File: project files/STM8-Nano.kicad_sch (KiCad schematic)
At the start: 29 parts, among them J1 RIGHT, J2 LEFT, J3 USB_C_Receptacle, J4 SWIM, SW1 RESET, SW2 VCC, U1 STM8F105K4, U2 CH340E, Y1 16MHZ

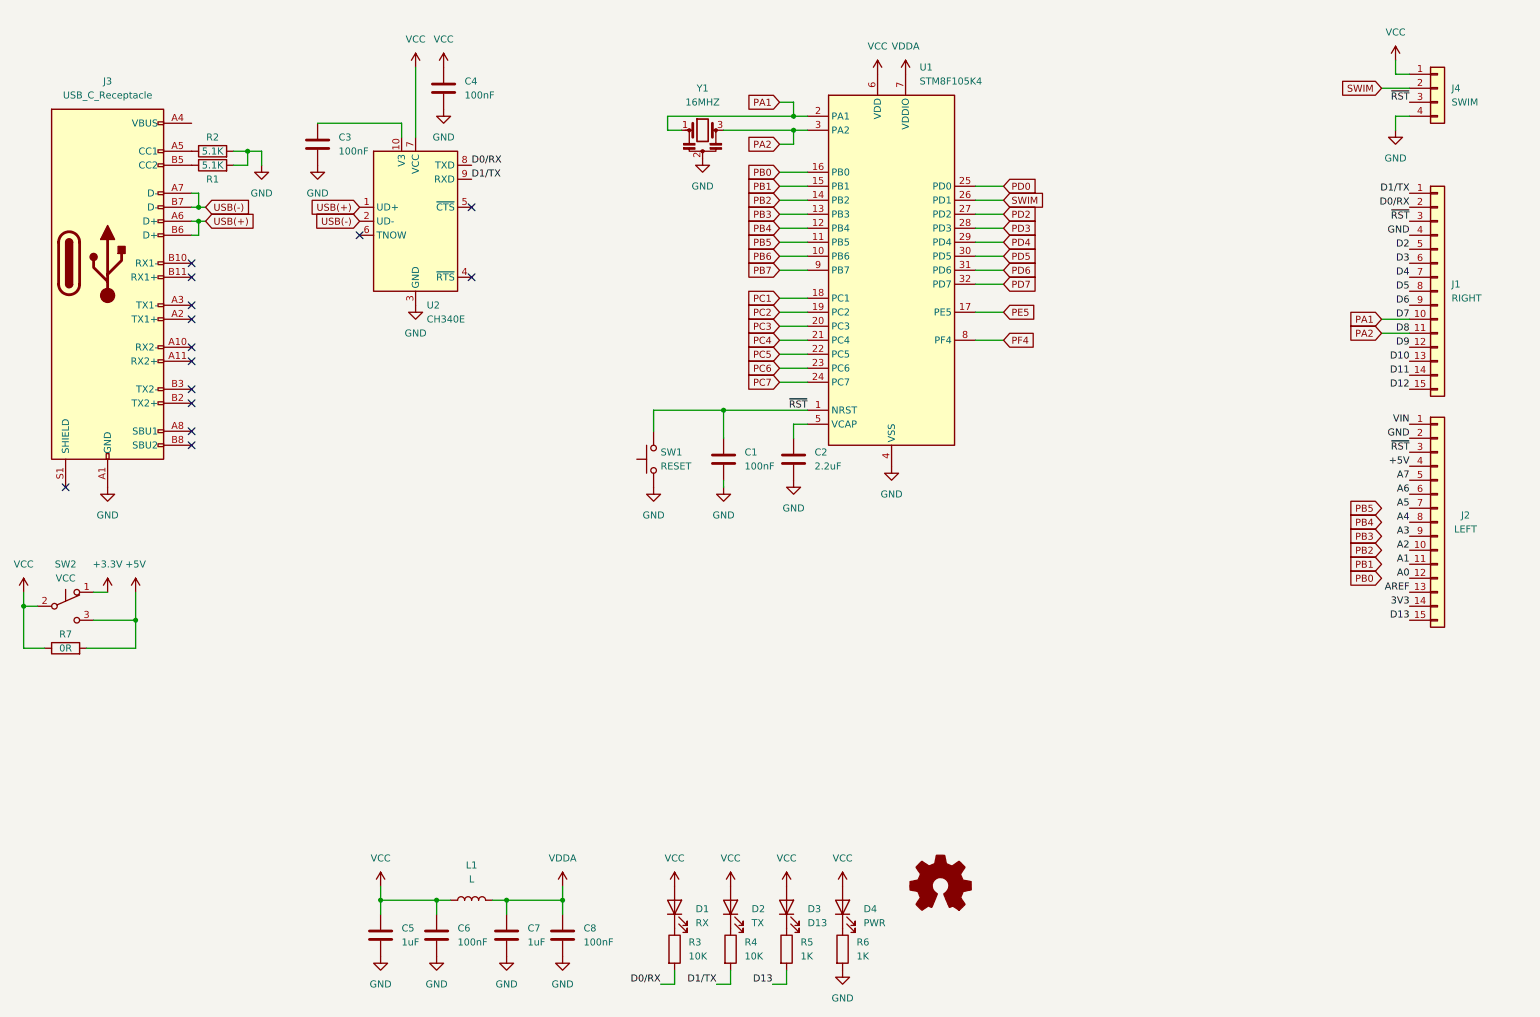
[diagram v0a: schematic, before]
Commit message: added annotation
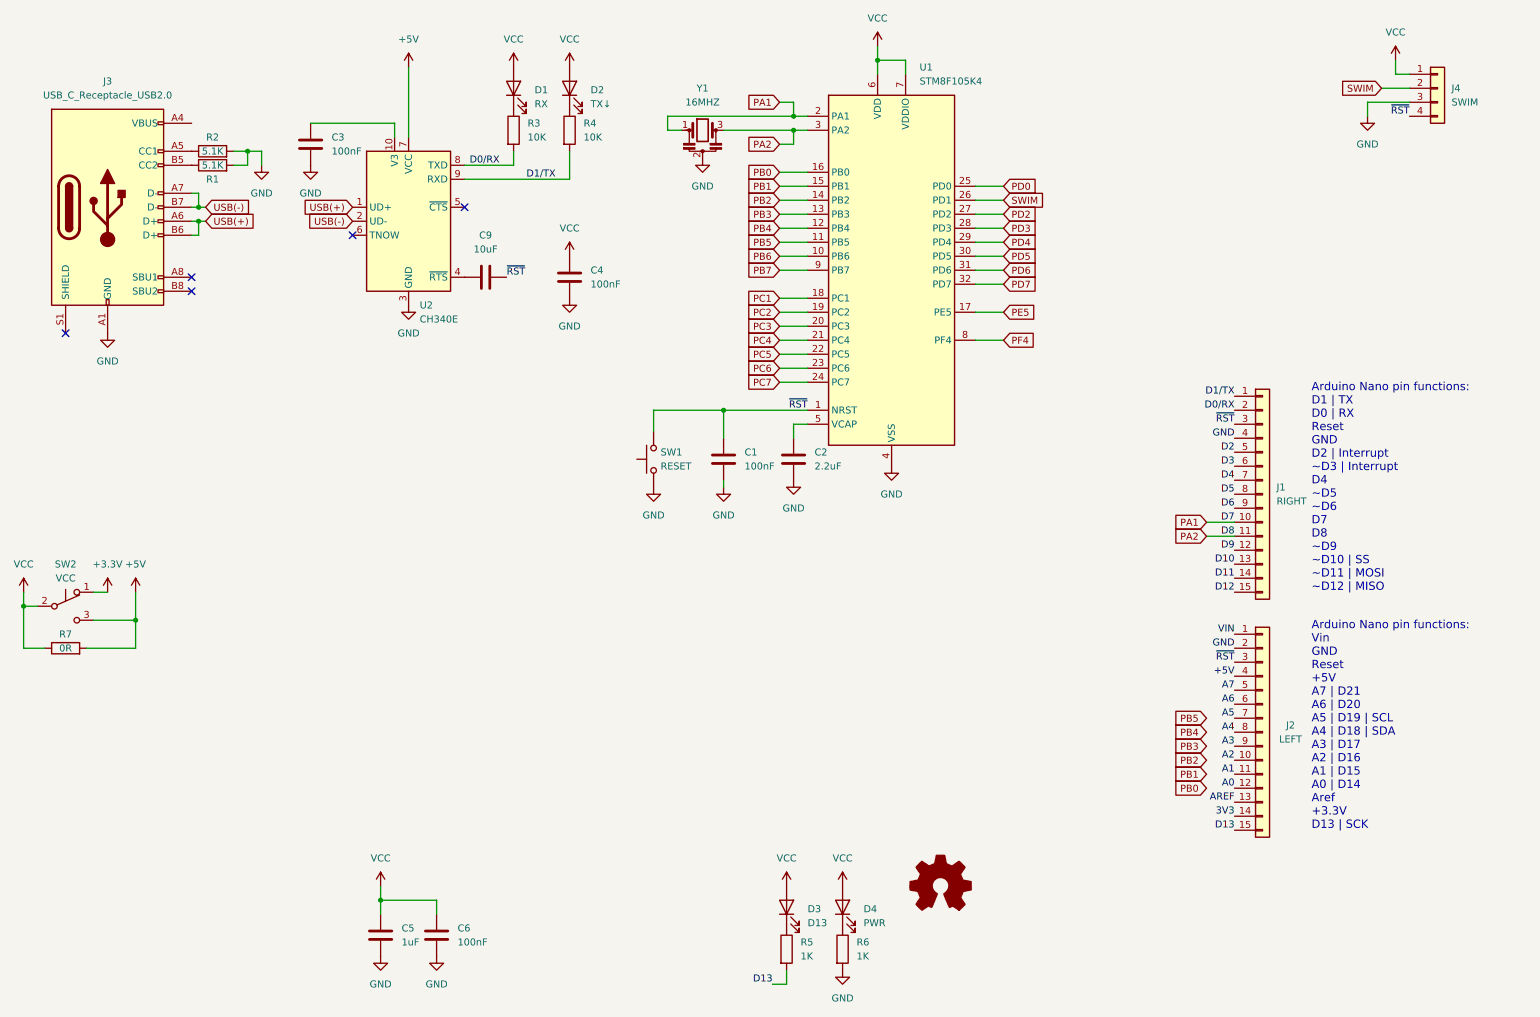
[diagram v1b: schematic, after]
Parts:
- removed C7: 1uF, Capacitor_SMD:C_0603_1608Metric, symbol Device:C
- removed C8: 100nF, Capacitor_SMD:C_0603_1608Metric, symbol Device:C
- removed J3: USB_C_Receptacle, Connector_USB:USB_C_Receptacle_Palconn_UTC16-G, symbol Connector:USB_C_Receptacle
- removed L1: L, symbol Device:L
- added C9: 10uF, Capacitor_SMD:C_0603_1608Metric, symbol Device:C
- added J3: USB_C_Receptacle_USB2.0, Connector_USB:USB_C_Receptacle_Palconn_UTC16-G, symbol Connector:USB_C_Receptacle_USB2.0
- D2: value TX -> TX↓
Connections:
- net VDDA is gone; now on net VCC: U1.7 (VDDIO)
- net +5V: now also U2.7 (VCC)
- net GND: now also J4.3 (Pin_3), J3.A1 (GND), J3.A12 (GND), J3.B1 (GND), J3.B12 (GND); no longer J4.4 (Pin_4)
- net USB(+): now also J3.A6 (D+), J3.B6 (D+)
- net USB(-): now also J3.A7 (D-), J3.B7 (D-)
- net VCC: no longer U2.7 (VCC)
- net ~{RST}: now also J4.4 (Pin_4), C9.2; no longer J4.3 (Pin_3)
- net at R1.1: now also J3.B5 (CC2)
- net at R2.1: now also J3.A5 (CC1)
- net at U2.4 (~{RTS}): now also C9.1
- new net: J3.A4 (VBUS), J3.A9 (VBUS), J3.B4 (VBUS), J3.B9 (VBUS)
- no-connect marks 14 -> 5
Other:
- note added: "Arduino Nano pin functions: D1 | TX D0 | RX Reset GND D2 | Interrupt ~D3 | Interrupt D4 ~D5 ~D6 D7 D8 ~D9 ~D10 | SS ~D11 | MOSI ~D12 | MISO"
- note added: "Arduino Nano pin functions: Vin GND Reset +5V A7 | D21 A6 | D20 A5 | D19 | SCL A4 | D18 | SDA A3 | D17 A2 | D16 A1 | D15 A0 | D14 Aref +3.3V D13 | SCK"
- moved on the sheet: C3, C4, D1, D2, J1, J2, R3, R4, U2
